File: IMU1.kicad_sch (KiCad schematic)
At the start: 6 parts, among them U1 262-BMI088

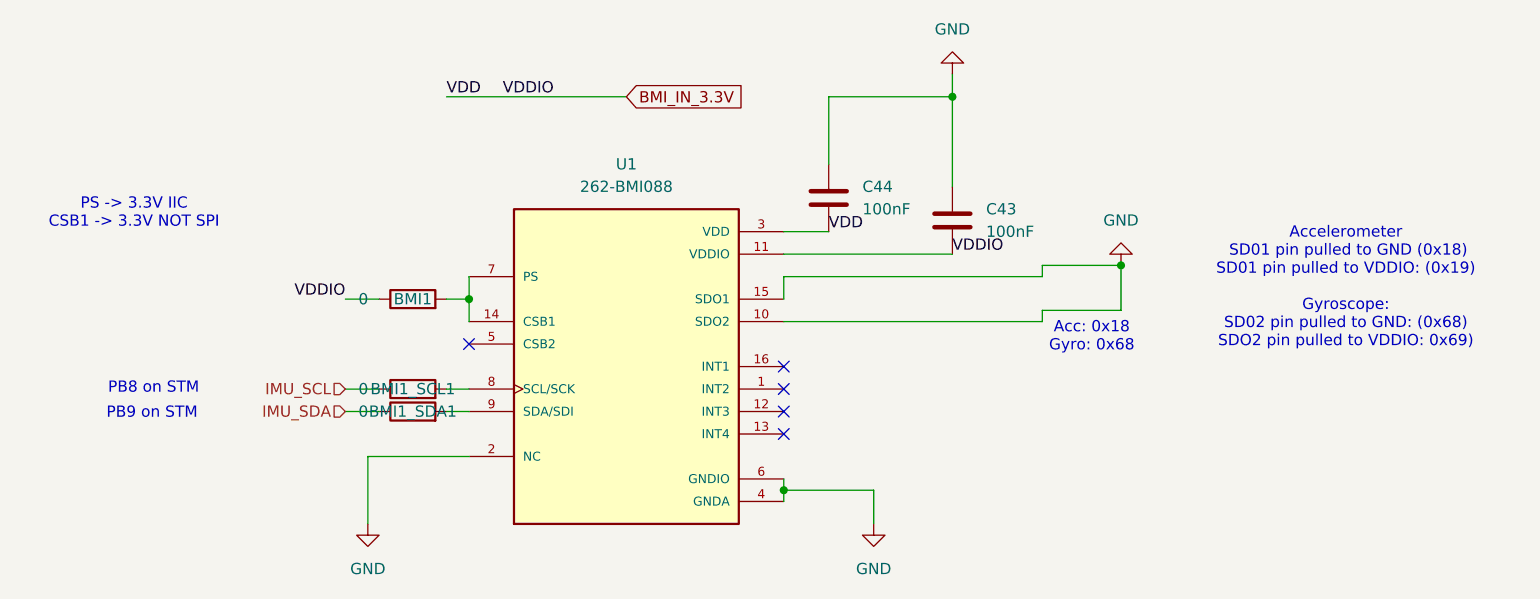
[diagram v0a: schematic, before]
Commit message: chore: Many routing changes
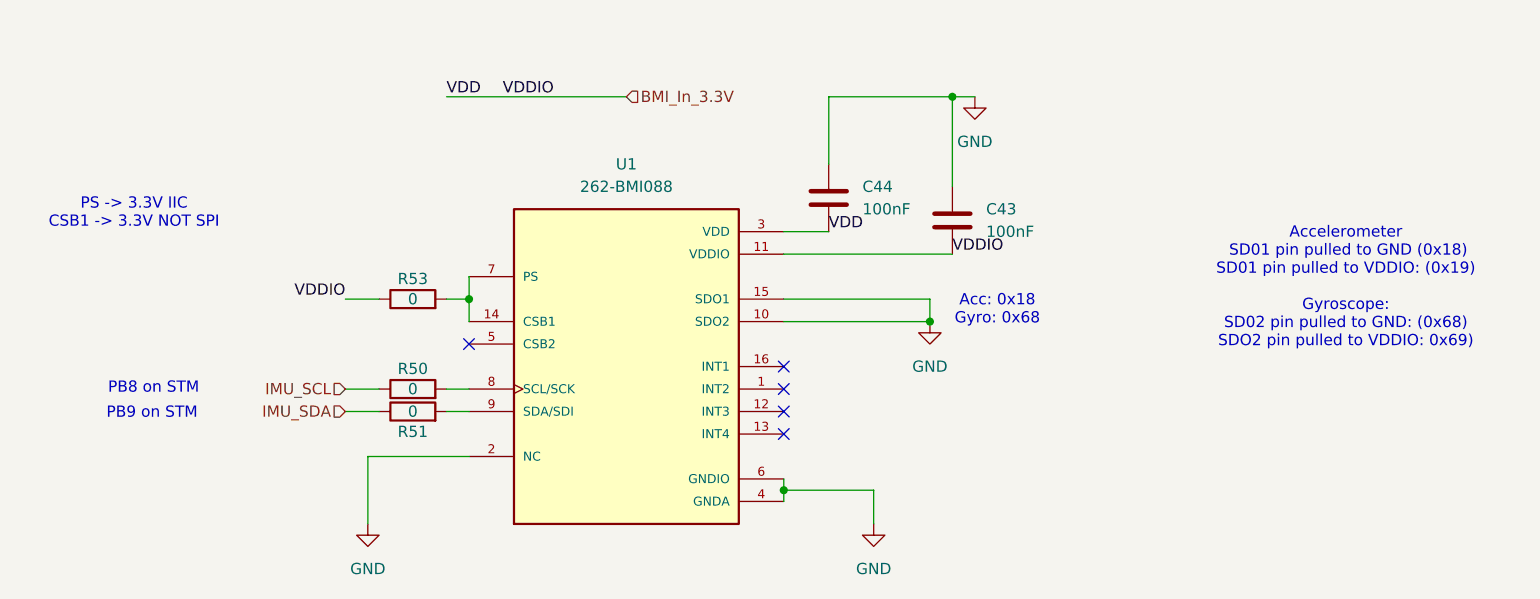
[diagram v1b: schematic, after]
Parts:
- removed BMI1, BMI1_SCL1, BMI1_SDA1: 0, Resistor_SMD:R_0603_1608Metric, symbol #dzdb:g_res/R-0-0603
- added R50, R51, R53: 0, Resistor_SMD:R_0603_1608Metric, symbol #dzdb:g_res/R-0-0603
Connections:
- net IMU_SCL: now also R50.1
- net IMU_SDA: now also R51.1
- net at U1.14 (CSB1), U1.7 (PS): now also R53.2
- net at U1.8 (SCL/SCK): now also R50.2
- net at U1.9 (SDA/SDI): now also R51.2
- net BMI_IN_3.3V renamed BMI_In_3.3V
- net BMI_In_3.3V: now also R53.1
